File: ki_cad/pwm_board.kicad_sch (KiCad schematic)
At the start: 5 parts, among them J10 Conn_01x04_Pin

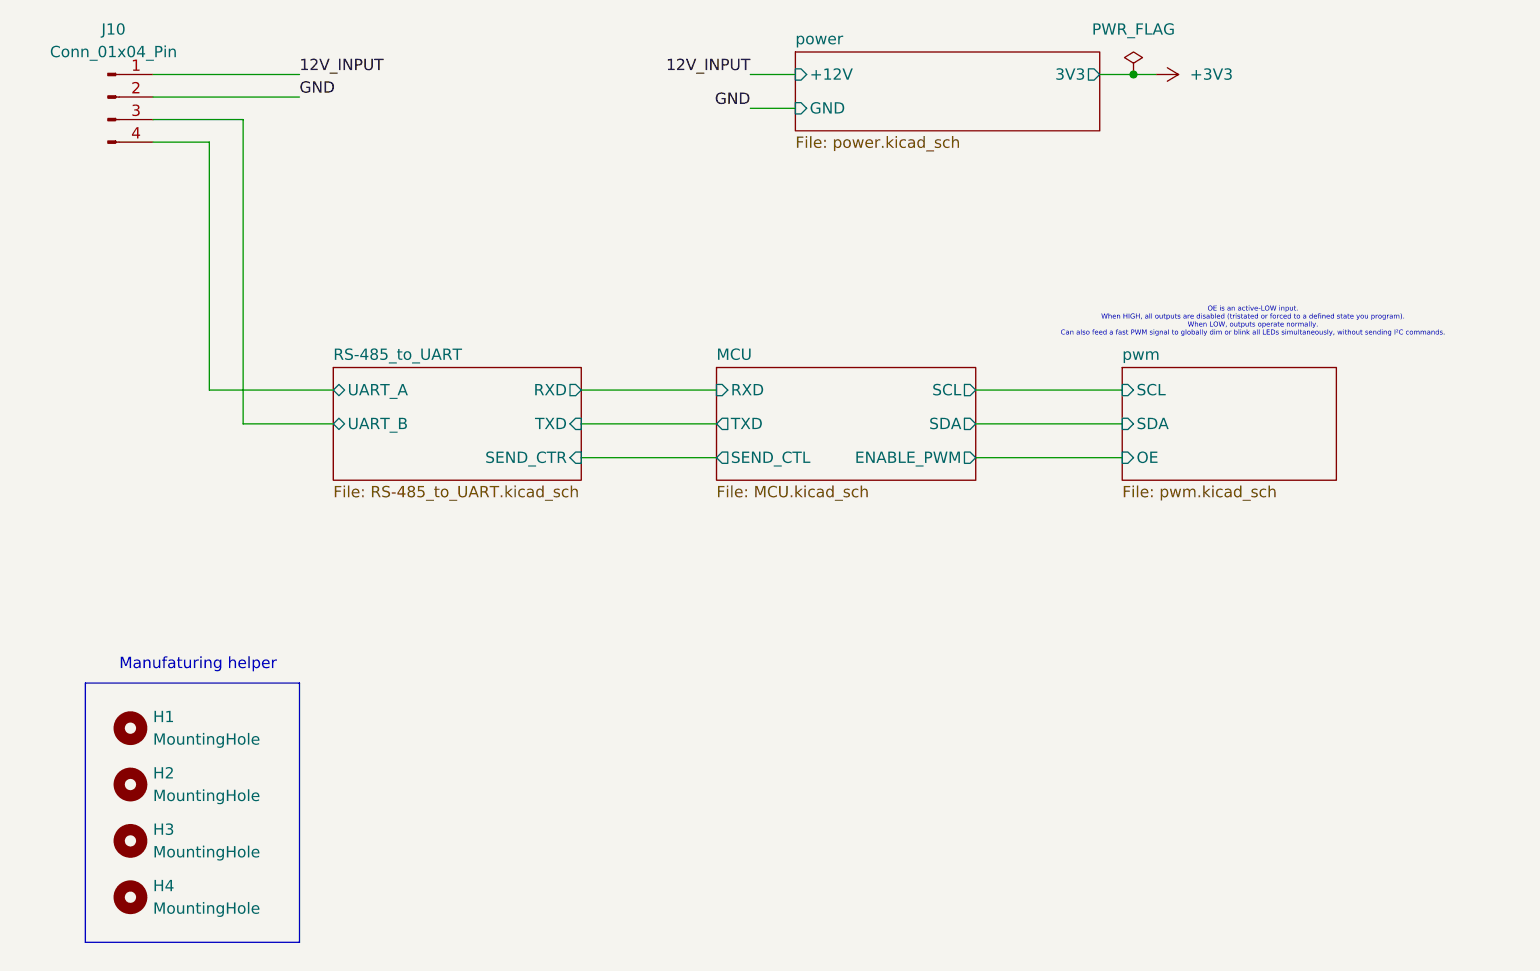
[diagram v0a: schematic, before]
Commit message: update after feedback (purchased)
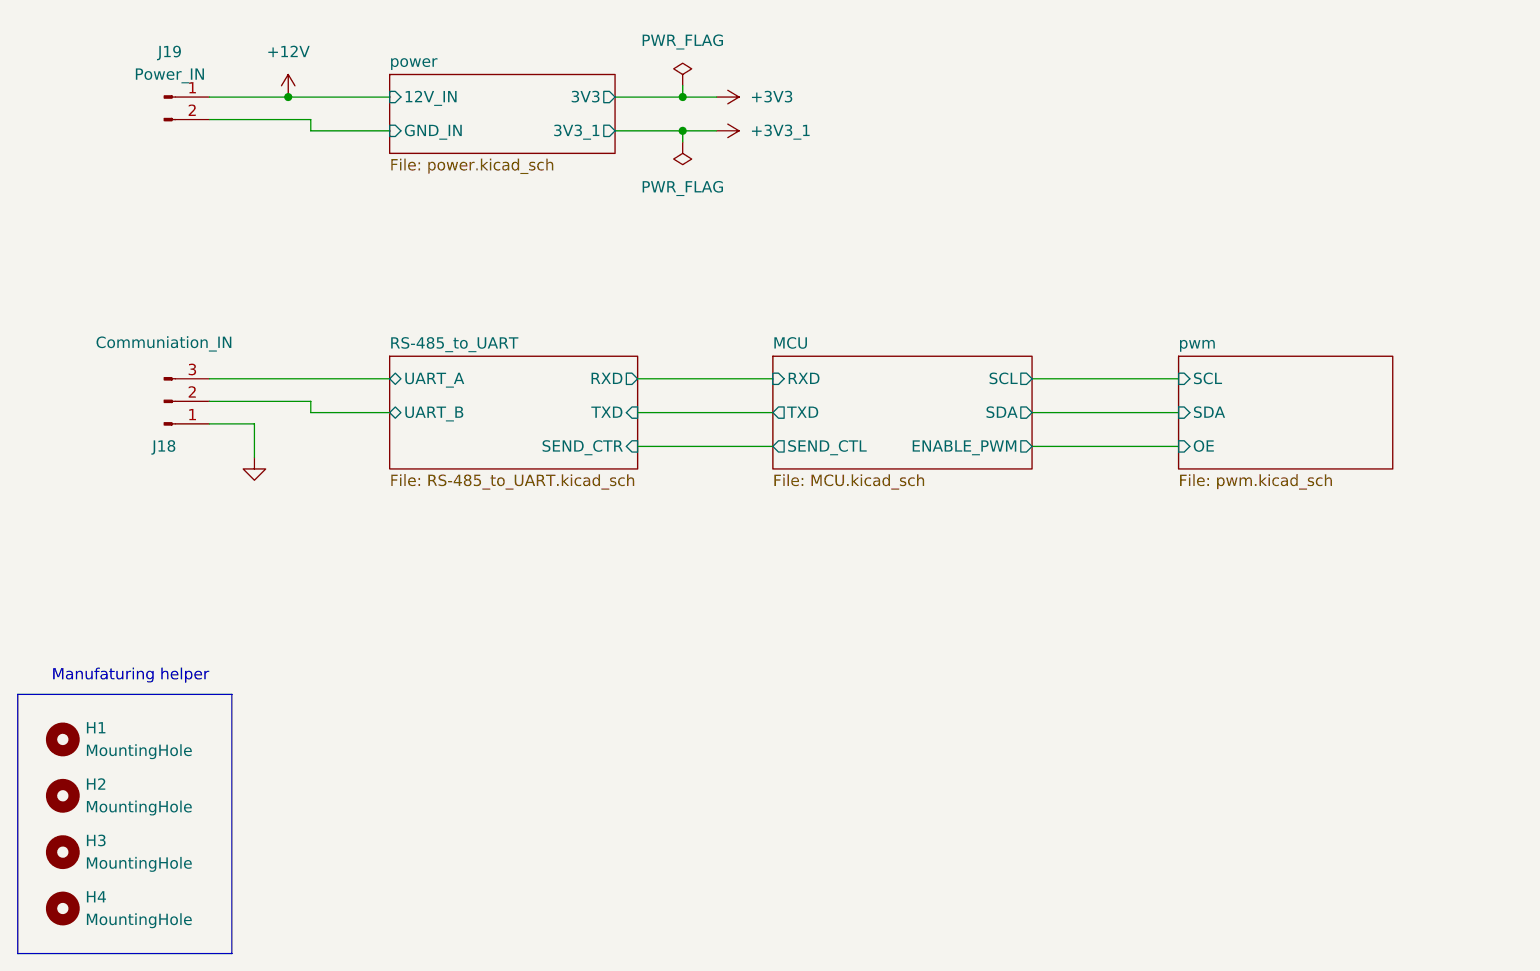
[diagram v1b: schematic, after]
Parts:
- removed J10: Conn_01x04_Pin, Connector_PinHeader_2.54mm:PinHeader_1x04_P2.54mm_Vertical, symbol Connector:Conn_01x04_Pin
- added J18: Communiation_IN, Connector_PinHeader_2.54mm:PinHeader_1x03_P2.54mm_Vertical, symbol Connector:Conn_01x03_Pin
- added J19: Power_IN, TerminalBlock:TerminalBlock_MaiXu_MX126-5.0-02P_1x02_P5.00mm, symbol Connector:Conn_01x02_Pin
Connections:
- net GND: now also J18.1 (Pin_1)
- net RS-485_to_UART/UART_A: now also J18.3 (Pin_3)
- net RS-485_to_UART/UART_B: now also J18.2 (Pin_2)
- new net +12V: J19.1 (Pin_1)
- new net power/GND_IN: J19.2 (Pin_2)
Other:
- sheet power ports: added 12V_IN, 3V3_1, GND_IN; removed +12V, GND
- note removed: "OE is an active‑LOW input. When HIGH, all outputs are disabled (tristated or forced to a defined state you program). When LOW, outputs operate normally. Can also feed a fast PWM signal to globally dim or blink all LEDs simultaneously, without sending I²C commands."
- moved on the sheet: H1, H2, H3
